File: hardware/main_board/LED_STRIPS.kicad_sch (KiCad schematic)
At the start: 9 parts, among them IC801 SN74LV1T34DBVR, J801 Conn_01x03_Pin, J802 Conn_01x03_Pin

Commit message: led info
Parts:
- C801: Mouser Price/Stock (none) -> https://www.mouser.com/ProductDetail/Samsung-Electro-Mechan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
- C802: Mouser Price/Stock (none) -> https://www.mouser.com/ProductDetail/Walsin/MG21B104K500CT?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
- U801: now left out of the parts list
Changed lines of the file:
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@@
+			)
+		)
+		(property "Mouser Price/Stock" "https://www.mouser.com/ProductDetail/Samsung-Electro-Mechanics/CL21A106KPFNNNE?qs=sGAEpiMZZMt7gvpyg0xT8jBAVP%252BdkPhuUJvUBe19zr8%3D"
+			(at 69.85 74.93 0)
+			(effects
+				(font
+					(size 1.27 1.27)
+				)
+				(hide yes)
 			)
 		)
@@
 		(unit 1)
 		(exclude_from_sim no)
-		(in_bom yes)
+		(in_bom no)
 		(on_board no)
 		(dnp no)
@@
 			(effects
 				(font
+					(size 1.27 1.27)
+				)
+				(hide yes)
+			)
+		)
+		(property "Mouser Price/Stock" "https://www.mouser.com/ProductDetail/Walsin/MG21B104K500CT?qs=sGAEpiMZZMt7gvpyg0xT8jBHDtGZvLzXjlSfFWC8Jgc2tQbZi0zprA%3D%3D"
+			(at 52.07 53.34 90)
+			(effects
+				(font

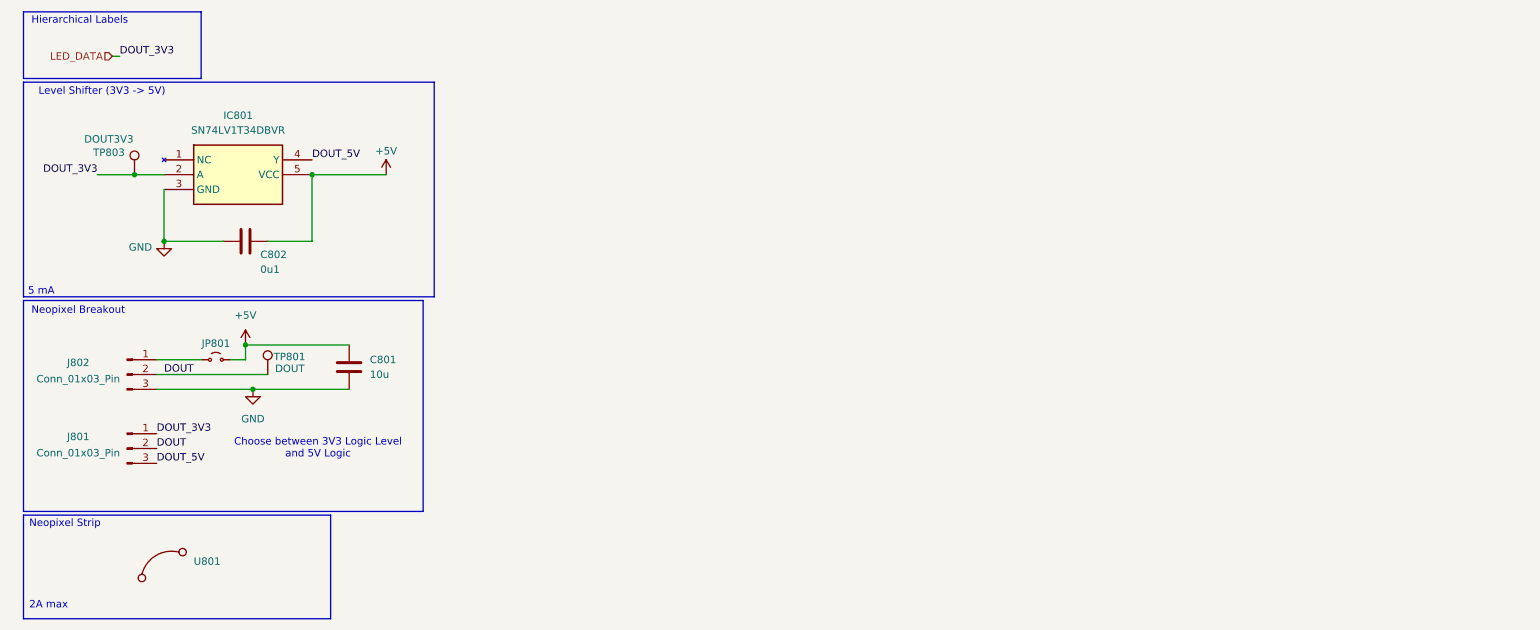
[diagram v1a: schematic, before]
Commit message: up to date scheamtic
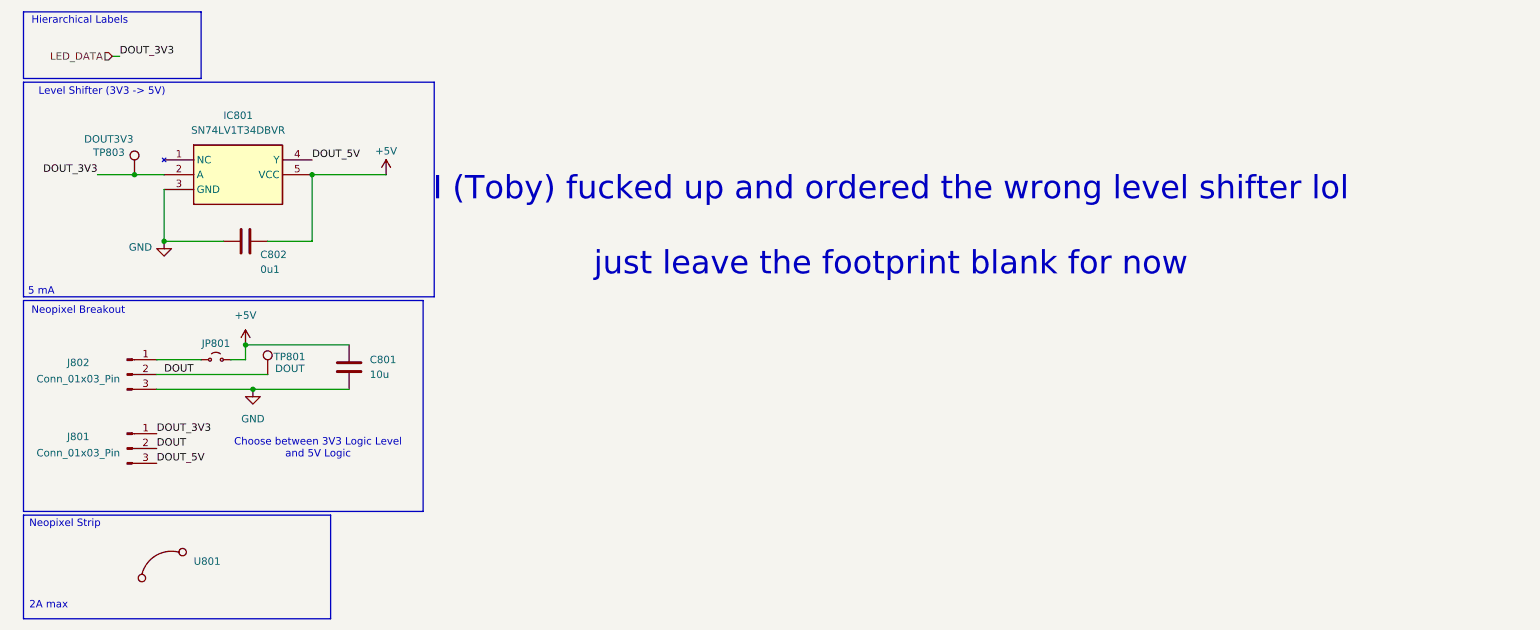
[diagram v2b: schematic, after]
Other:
- note added: "I (Toby) fucked up and ordered the wrong level shifter lol just leave the footprint blank for now"
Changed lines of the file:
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@@
+		)
+	)
+	(text "I (Toby) fucked up and ordered the wrong level shifter lol\n\njust leave the footprint blank for now"
+		(exclude_from_sim no)
+		(at 162.814 50.8 0)
+		(effects
+			(font
+				(size 4 4)
+				(color 255 0 32 1)
+			)
 		)
 	)

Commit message: kys harddare
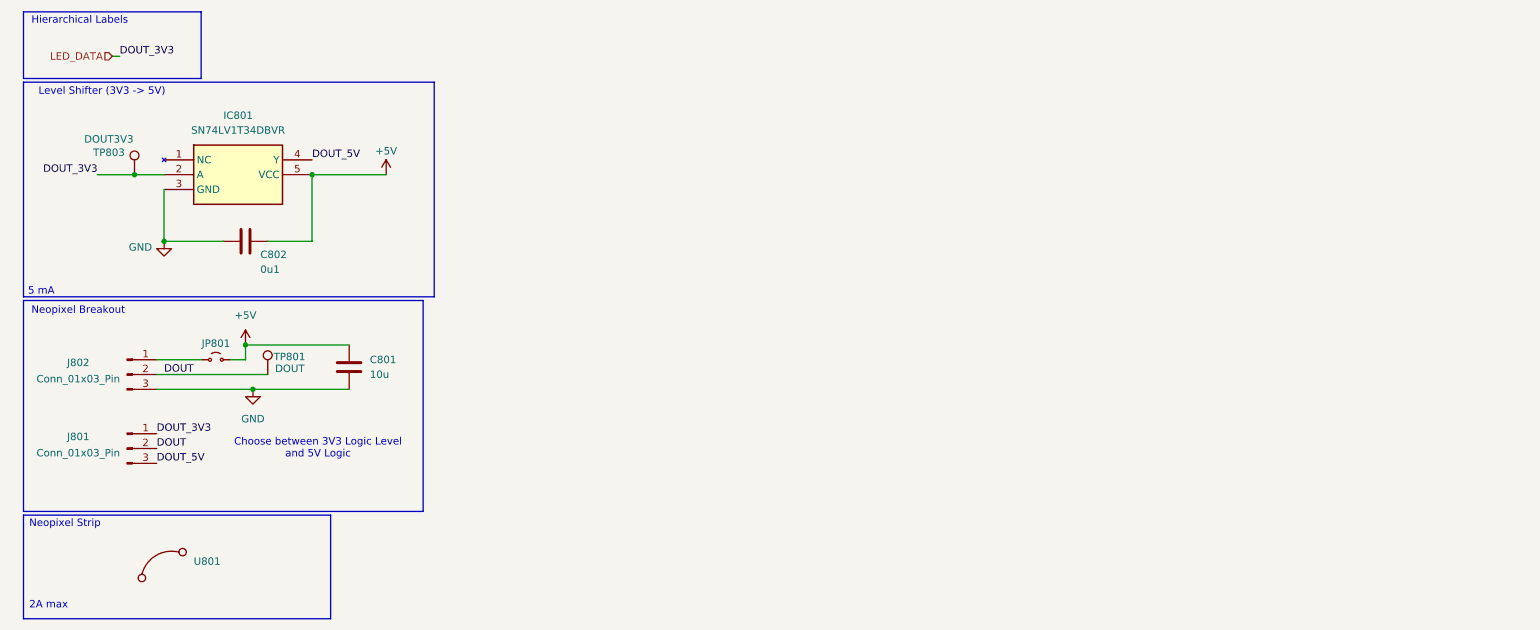
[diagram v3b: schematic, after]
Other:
- note removed: "I (Toby) fucked up and ordered the wrong level shifter lol just leave the footprint blank for now"
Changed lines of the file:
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@@
-		)
-	)
-	(text "I (Toby) fucked up and ordered the wrong level shifter lol\n\njust leave the footprint blank for now"
-		(exclude_from_sim no)
-		(at 162.814 50.8 0)
-		(effects
-			(font
-				(size 4 4)
-				(color 255 0 32 1)
-			)
 		)
 	)
